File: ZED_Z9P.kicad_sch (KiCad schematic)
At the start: 16 parts, among them IC2 ZED-F9P-05B

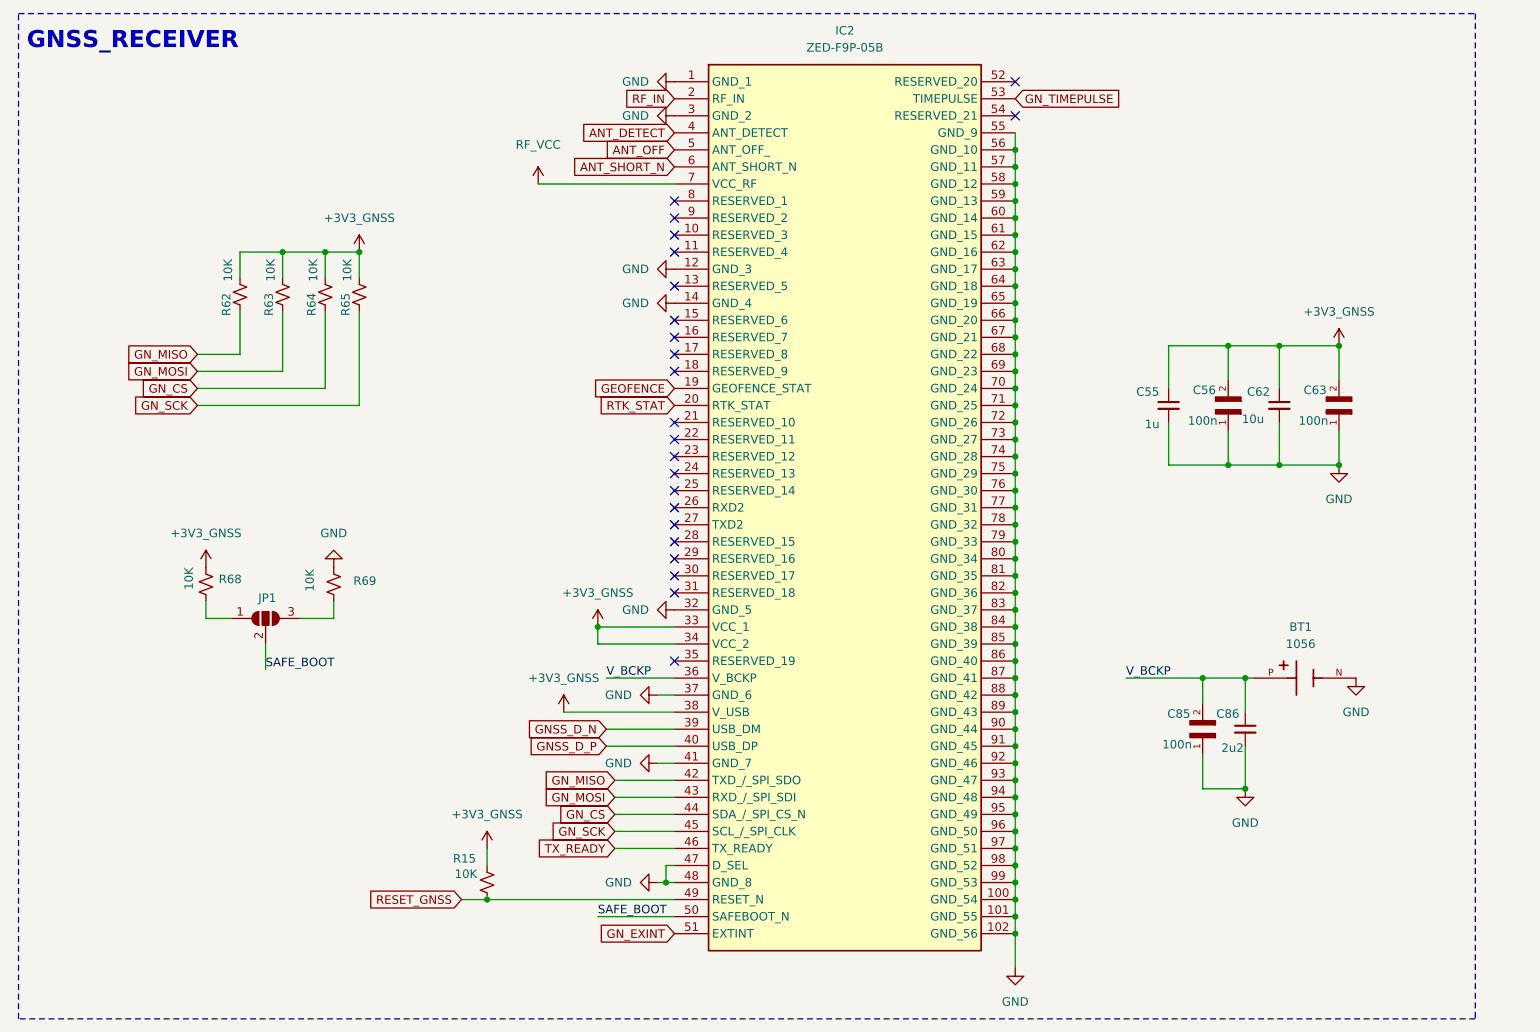
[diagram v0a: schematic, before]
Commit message: 123
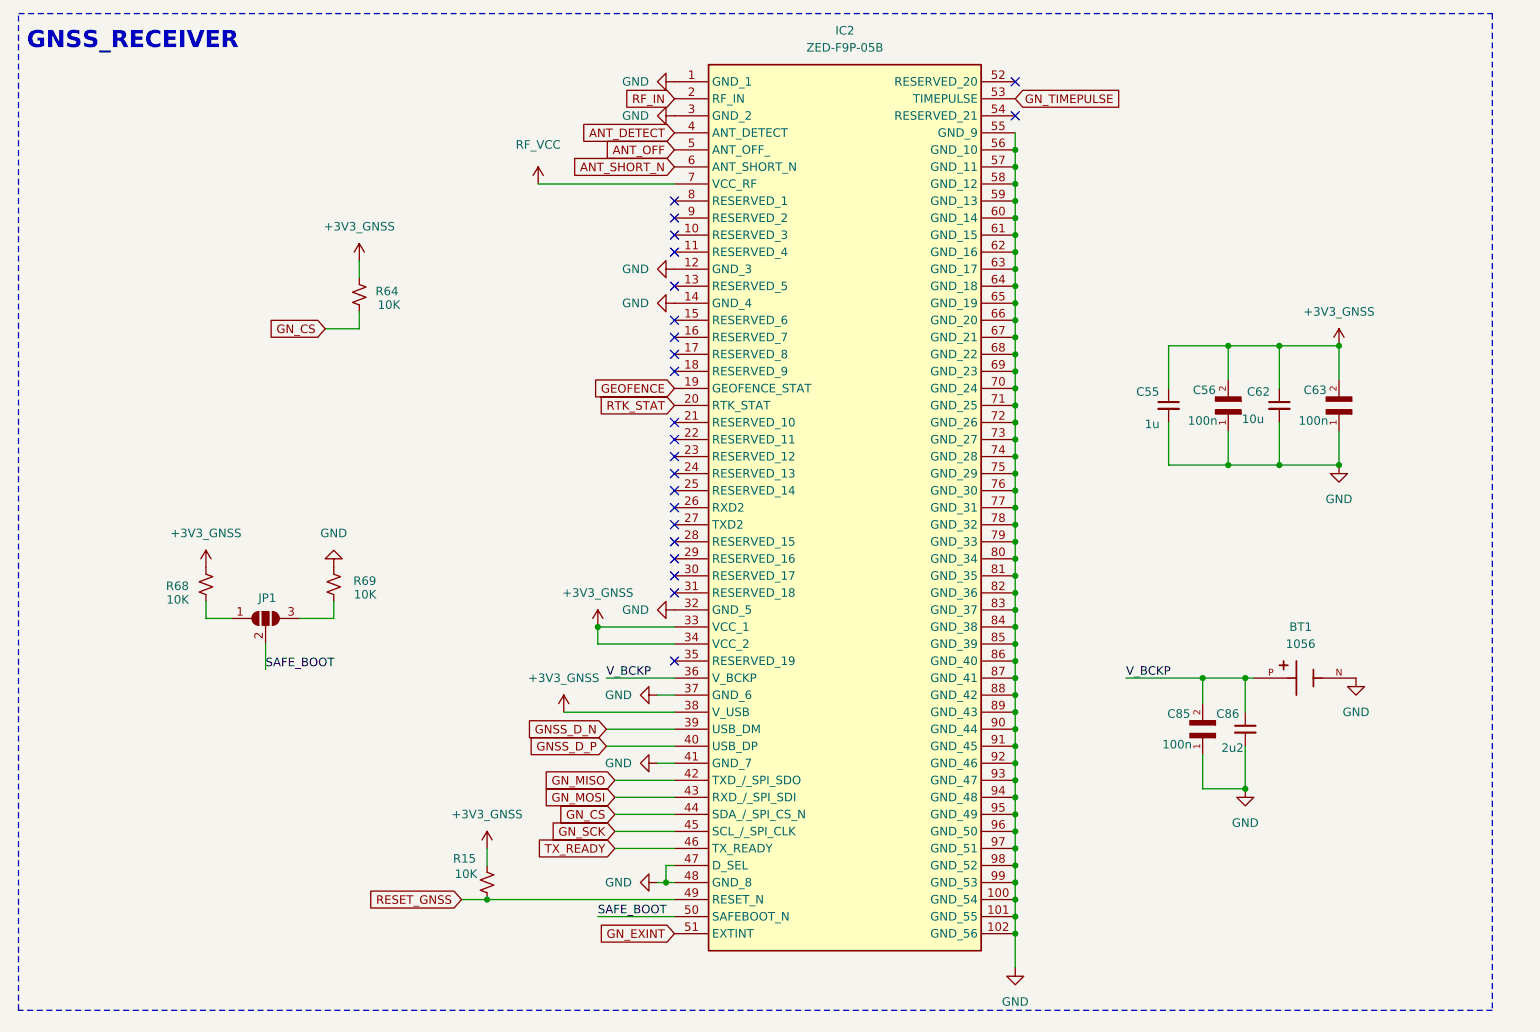
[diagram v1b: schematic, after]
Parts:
- removed R62, R63, R65: 10K, Resistor_SMD:R_0402_1005Metric, symbol Device:R_Small_US
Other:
- moved on the sheet: R64

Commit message: new
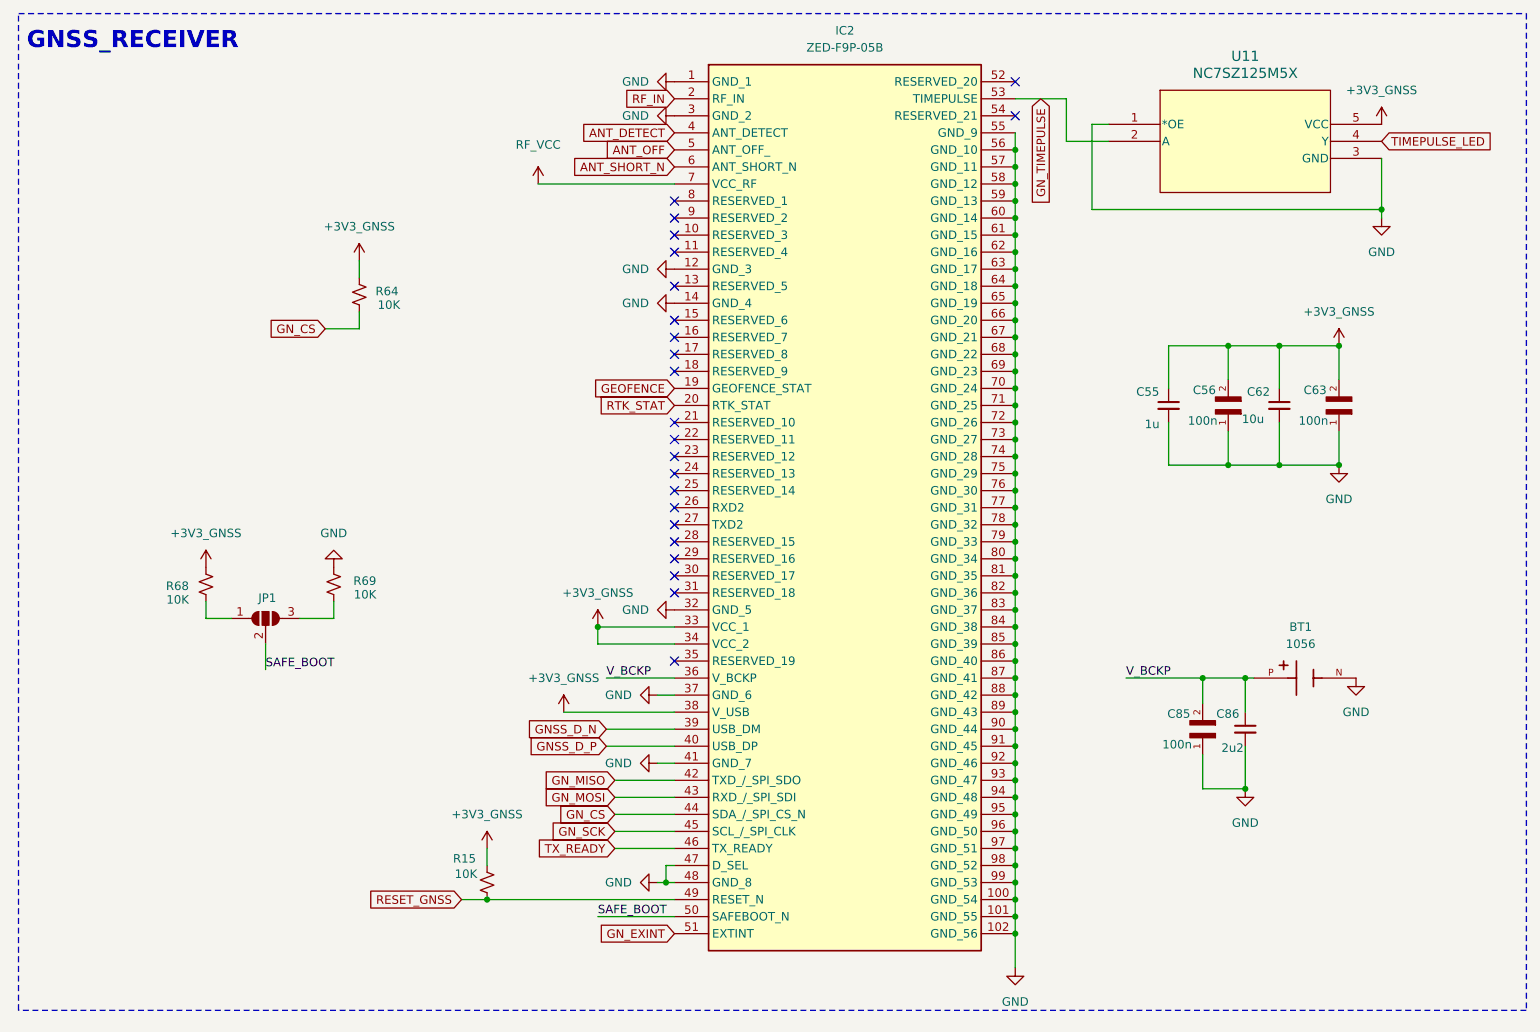
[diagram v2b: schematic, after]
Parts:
- added U11: NC7SZ125M5X, SC-74A_318BQ_ONS, symbol 2026-09-29_16-21-45:NC7SZ125M5X
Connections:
- net +3V3_GNSS: now also U11.5 (VCC)
- net GND: now also U11.1 (*OE), U11.3 (GND)
- net GN_TIMEPULSE: now also U11.2 (A)
- new net TIMEPULSE_LED: U11.4 (Y)
